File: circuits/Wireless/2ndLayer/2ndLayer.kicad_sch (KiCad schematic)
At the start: 21 parts, among them J1 Conn_01x10_Pin, J2 Conn_02x10_Odd_Even, Q16 BSS138, SW1 SW_SPST, U1 STM32F446RETx, Y1 16MHz

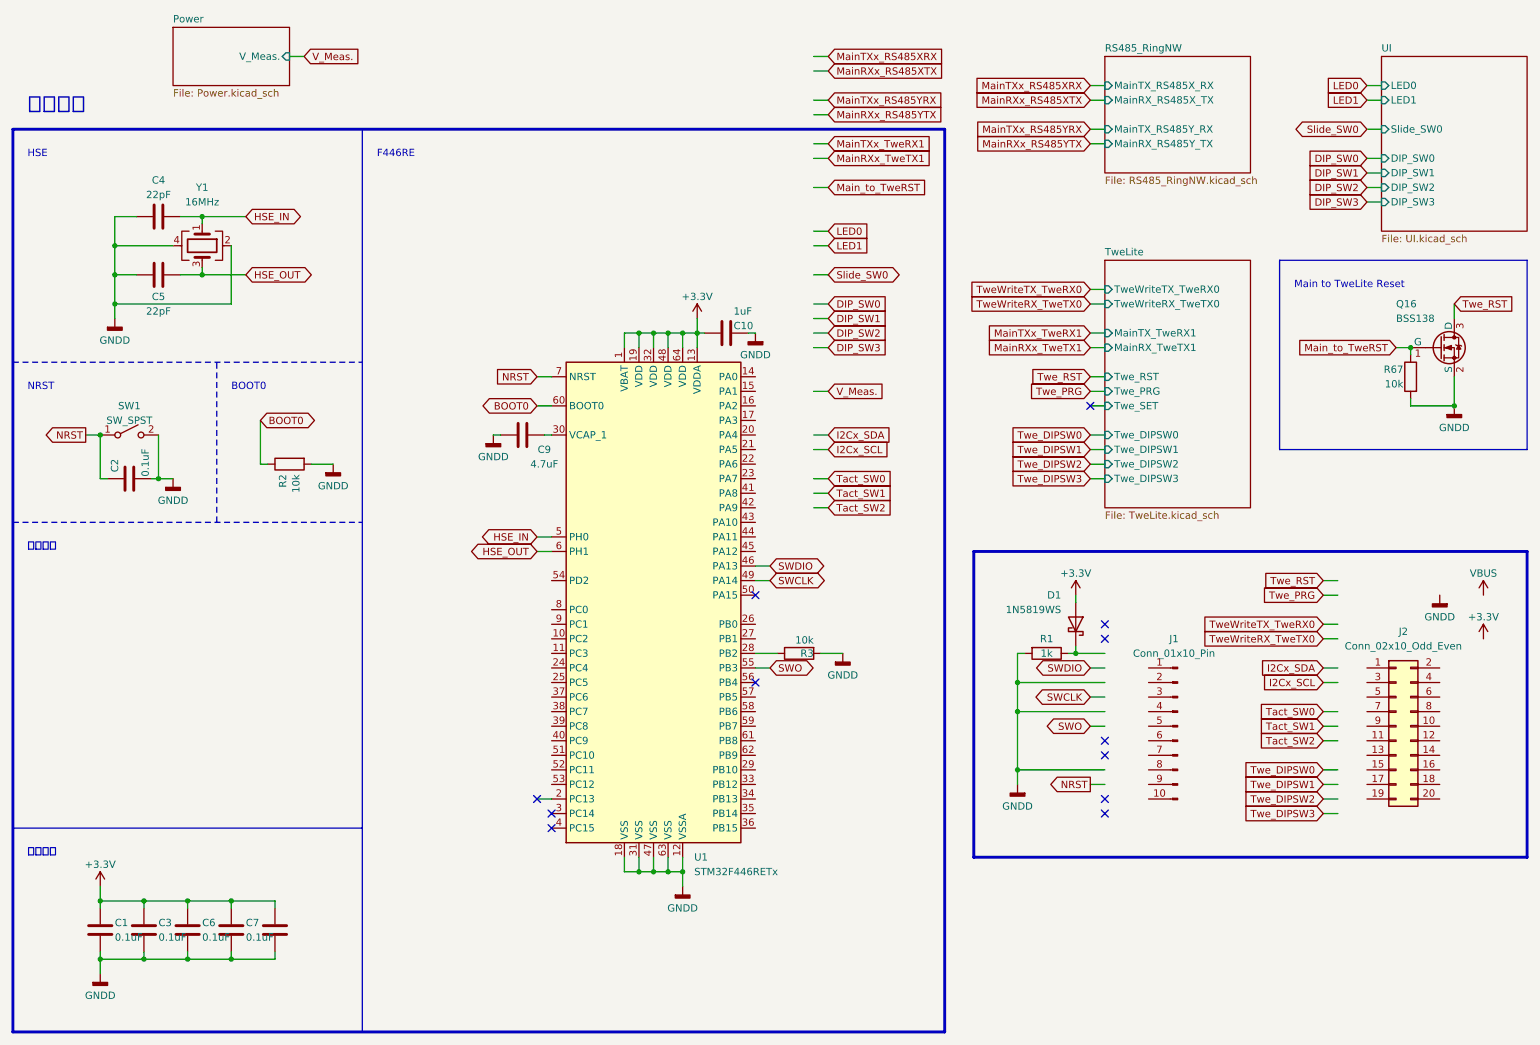
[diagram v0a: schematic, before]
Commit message: ラズパイ基板とか
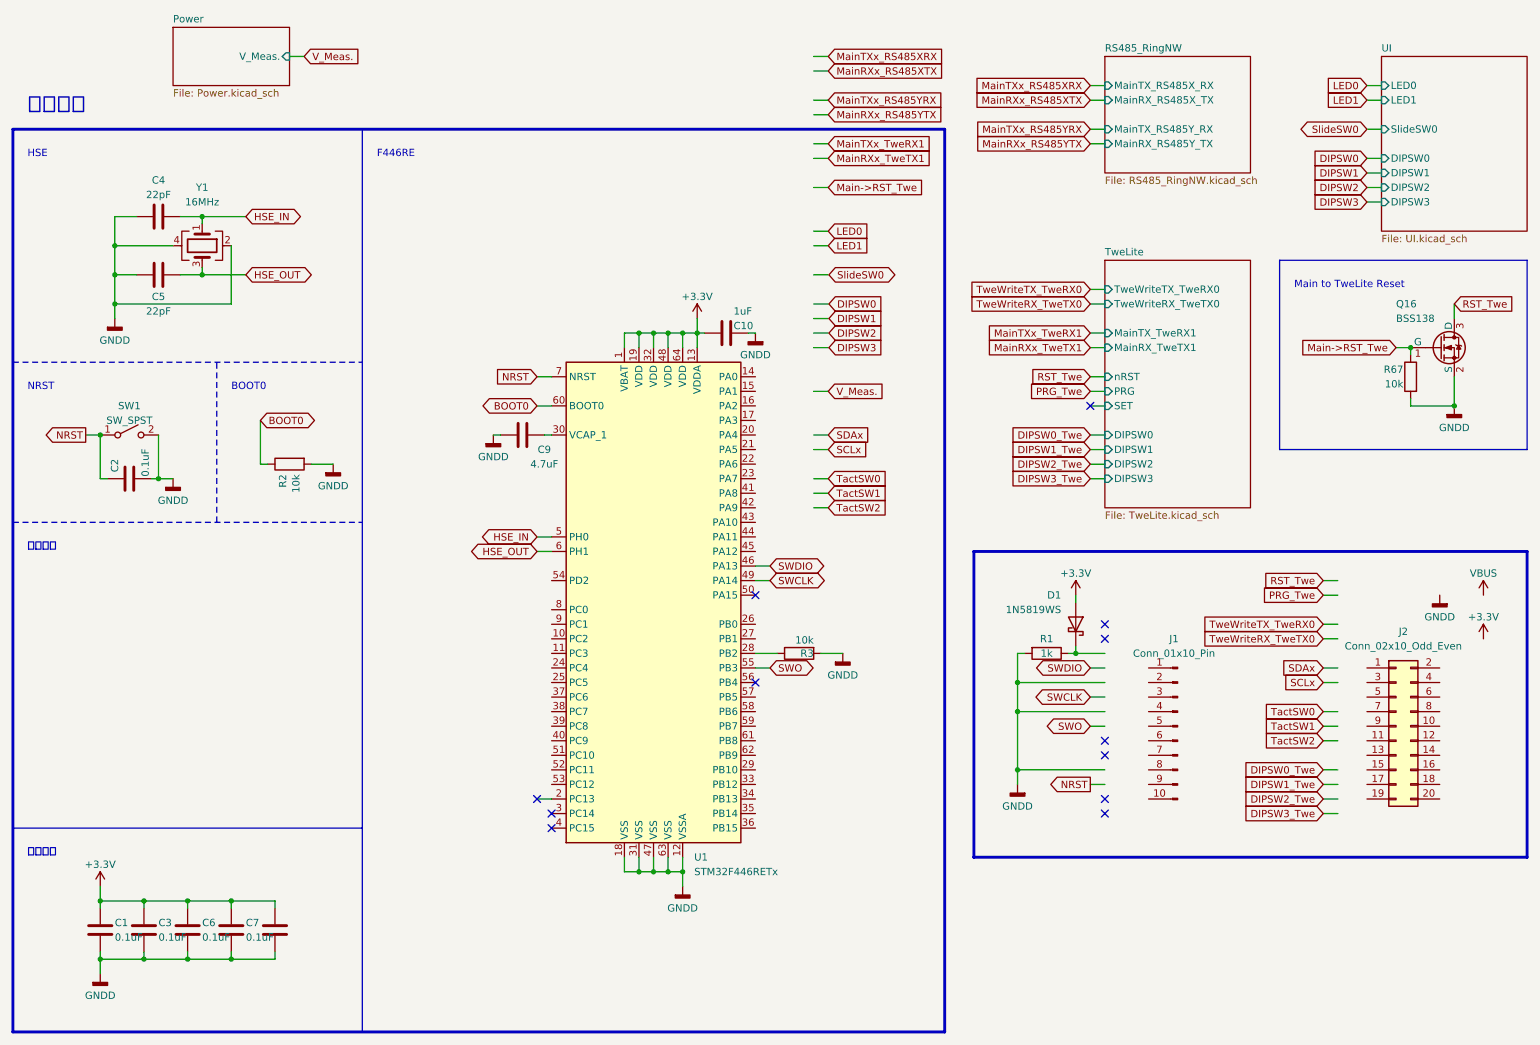
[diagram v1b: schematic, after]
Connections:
- net Main_to_TweRST renamed Main->RST_Twe
- net Twe_RST renamed RST_Twe
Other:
- sheet TweLite ports: added DIPSW0, DIPSW1, DIPSW2, DIPSW3, PRG, SET, nRST; removed Twe_DIPSW0, Twe_DIPSW1, Twe_DIPSW2, Twe_DIPSW3, Twe_PRG, Twe_RST, Twe_SET
- sheet UI ports: added DIPSW0, DIPSW1, DIPSW2, DIPSW3, SlideSW0; removed DIP_SW0, DIP_SW1, DIP_SW2, DIP_SW3, Slide_SW0

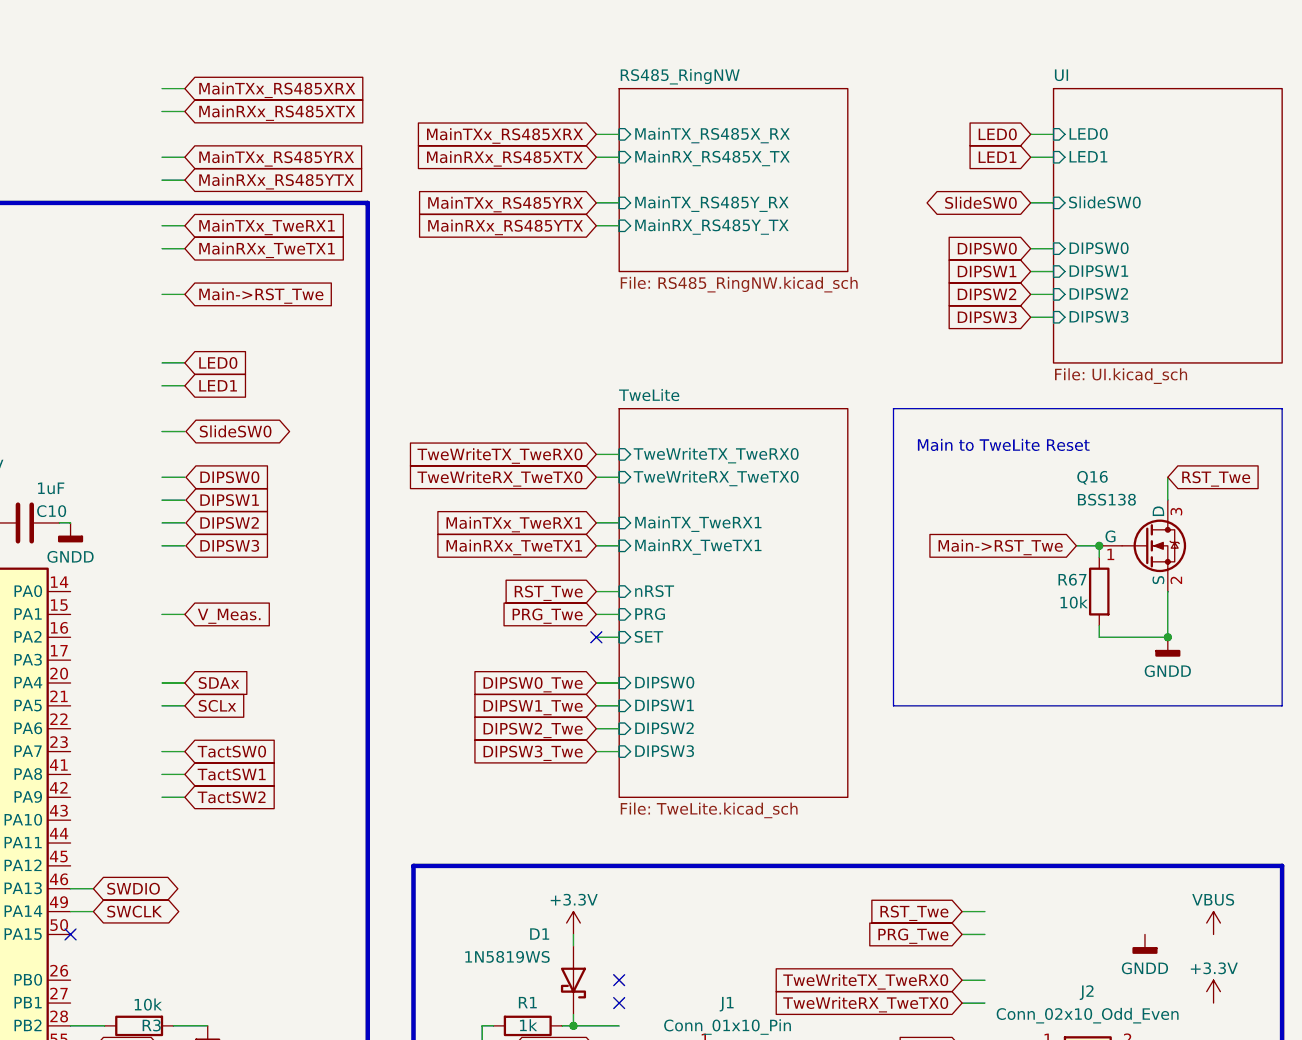
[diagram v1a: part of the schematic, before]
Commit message: PDFプロット
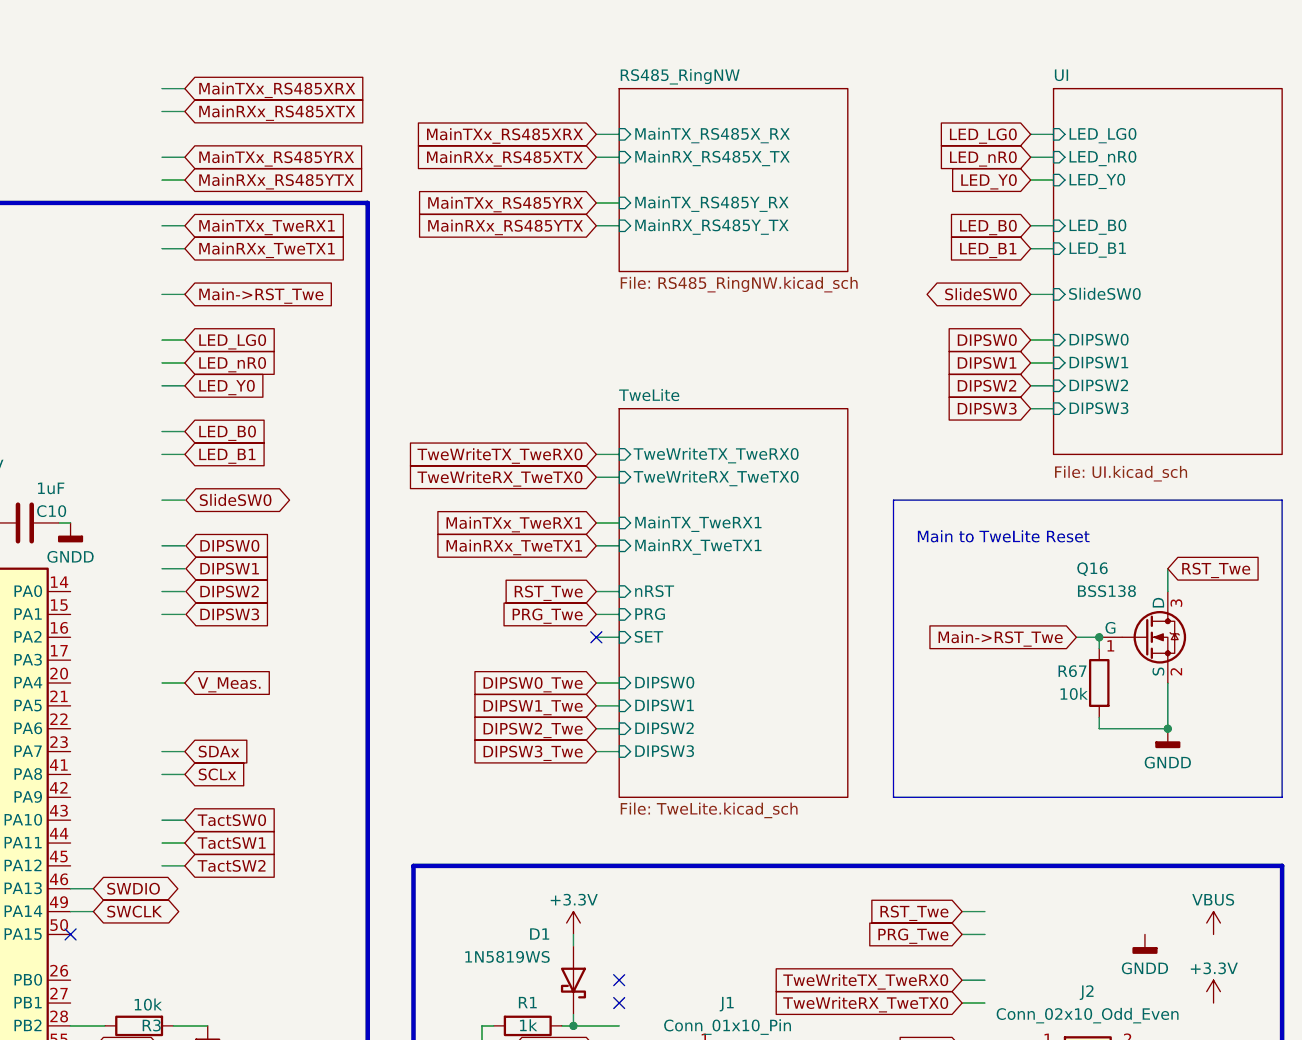
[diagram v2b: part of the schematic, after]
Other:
- sheet UI ports: added LED_B0, LED_B1, LED_LG0, LED_Y0, LED_nR0; removed LED0, LED1
- moved on the sheet: Q16, R67
